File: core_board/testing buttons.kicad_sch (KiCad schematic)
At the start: 45 parts, among them Q19 NMOS, Q2 PMOS, Q3 PMOS, Q4 PMOS, Q5 PMOS, Q6 PMOS, Q7 PMOS, Q8 PMOS, SW1 SW_Push, SW2 SW_Push, SW3 SW_Push, SW4 SW_Push

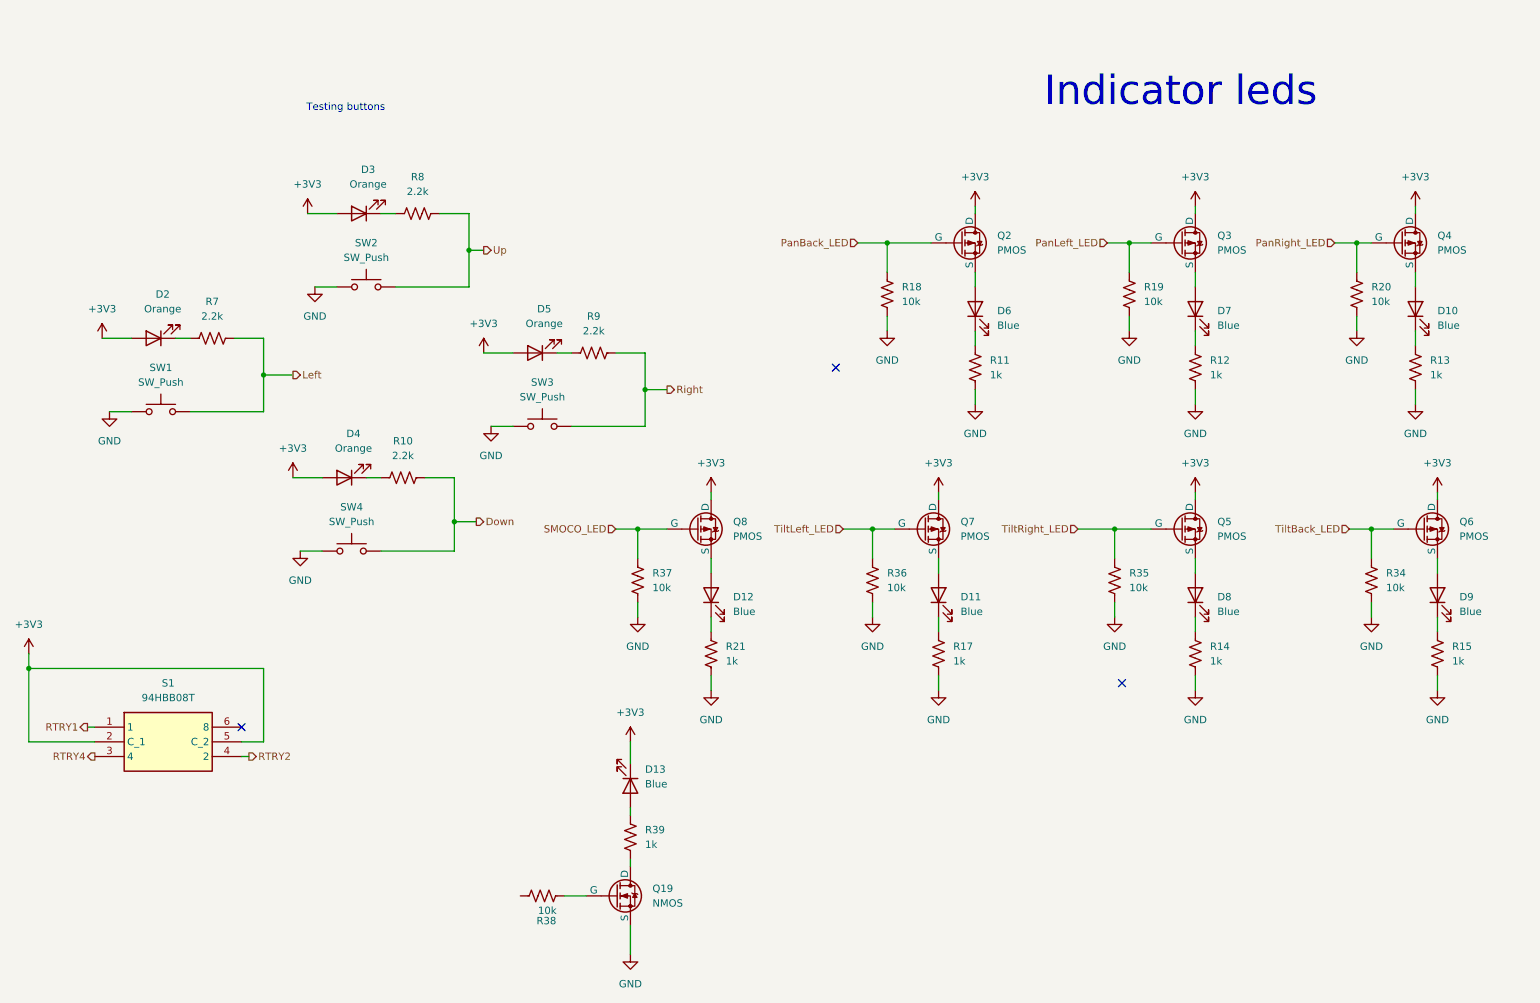
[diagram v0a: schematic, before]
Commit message: add
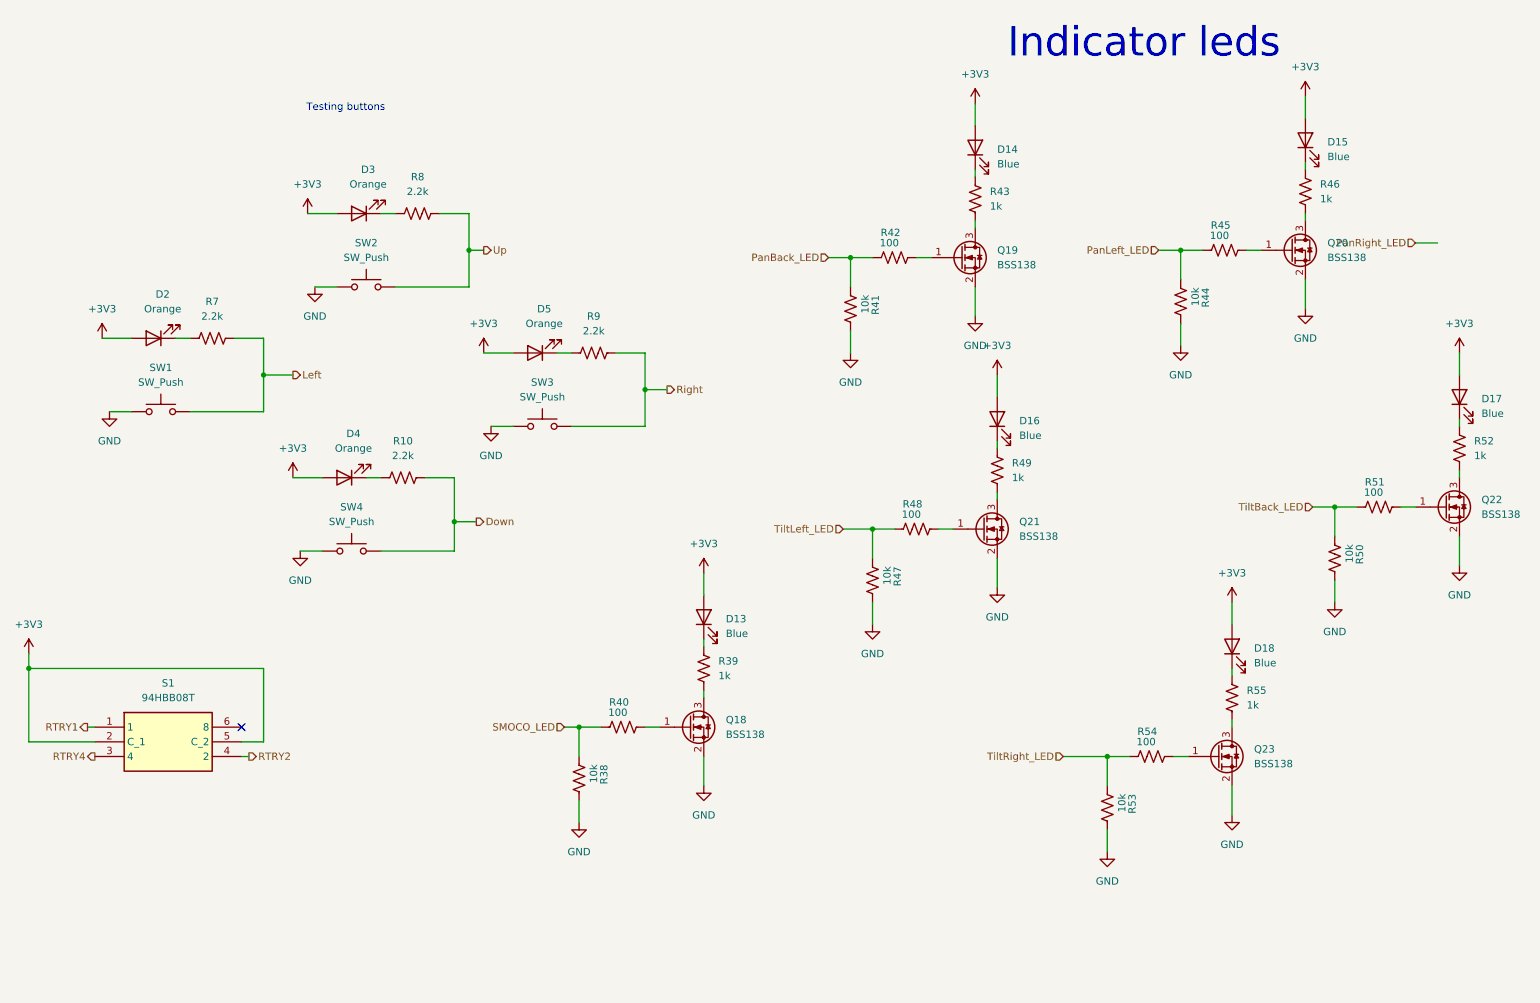
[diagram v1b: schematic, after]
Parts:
- removed D10, D11, D12, D6, D7, D8, D9: Blue, symbol Device:LED
- removed Q19: NMOS, symbol Simulation_SPICE:NMOS
- removed Q2, Q3, Q4, Q5, Q6, Q7, Q8: PMOS, symbol Simulation_SPICE:PMOS
- removed R11, R12, R13, R14, R15, R17, R21: 1k, symbol Device:R_US
- removed R18, R19, R20, R34, R35, R36, R37: 10k, symbol Device:R_US
- added D14, D15, D16, D17, D18: Blue, symbol Device:LED
- added Q18, Q19, Q20, Q21, Q22, Q23: BSS138, Package_TO_SOT_SMD:SOT-23, symbol Transistor_FET:BSS138
- added R40, R42, R45, R48, R51, R54: 100, symbol Device:R_US
- added R41, R44, R47, R50, R53: 10k, symbol Device:R_US
- added R43, R46, R49, R52, R55: 1k, symbol Device:R_US
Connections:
- net +3V3: now also D13.2 (A), D14.2 (A), D15.2 (A), D16.2 (A), D17.2 (A), D18.2 (A); no longer D13.1 (K)
- net GND: now also R38.2, Q18.2 (S), Q19.2 (S), Q20.2 (S), Q21.2 (S), Q22.2 (S), Q23.2 (S), R41.2, R44.2, R47.2, R50.2, R53.2
- net PanBack_LED: now also R41.1, R42.1
- net PanLeft_LED: now also R44.1, R45.1
- net SMOCO_LED: now also R38.1, R40.1
- net TiltBack_LED: now also R50.1, R51.1
- net TiltLeft_LED: now also R47.1, R48.1
- net TiltRight_LED: now also R53.1, R54.1
- net at R39.1: now also D13.1 (K); no longer D13.2 (A)
- net at R39.2: now also Q18.3 (D)
- new net: D14.1 (K), R43.1
- new net: D15.1 (K), R46.1
- new net: Q19.3 (D), R43.2
- new net: Q19.1 (G), R42.2
- new net: Q22.1 (G), R51.2
- new net: Q22.3 (D), R52.2
- new net: Q20.3 (D), R46.2
- new net: Q23.1 (G), R54.2
- new net: D17.1 (K), R52.1
- new net: D16.1 (K), R49.1
- new net: Q21.3 (D), R49.2
- new net: Q18.1 (G), R40.2
- new net: Q20.1 (G), R45.2
- new net: Q21.1 (G), R48.2
- new net: D18.1 (K), R55.1
- new net: Q23.3 (D), R55.2
- no-connect marks 3 -> 1
